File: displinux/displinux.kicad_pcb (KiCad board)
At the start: 2 copper layers, 145 parts, among them J1 USB4105-GF-A, J10 Conn_01x03, J2 USB4105-GF-A, J3 AudioJack4, J4 Conn_02x10_Counter_Clockwise, J5 HR911105A, J6 Conn_01x24_MountingPin, J7 Conn_01x06, J8 Conn_01x40_MountingPin, J9 Conn_01x02_Pin, U1 DP83848C, U2 SY8089AAAC, U3 F133, U4 SY8089AAAC, U5 XC6206P_2_8_MR, U6 XC6206P_1_2_MR, U7 SY7201ABC, U8 W25N01KV, X1 ASE-50MHz, Y1 24M, Y2 Crystal

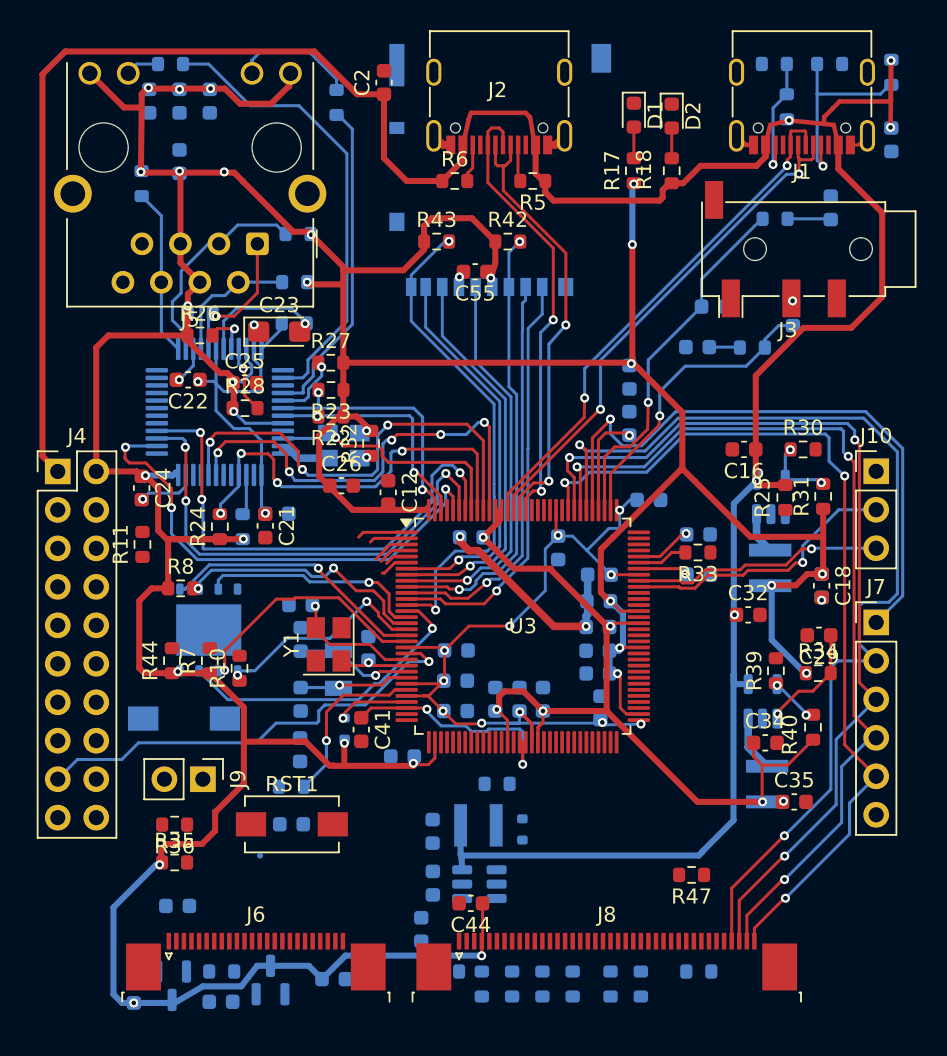
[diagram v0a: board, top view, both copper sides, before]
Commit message: tracing finished Need to check
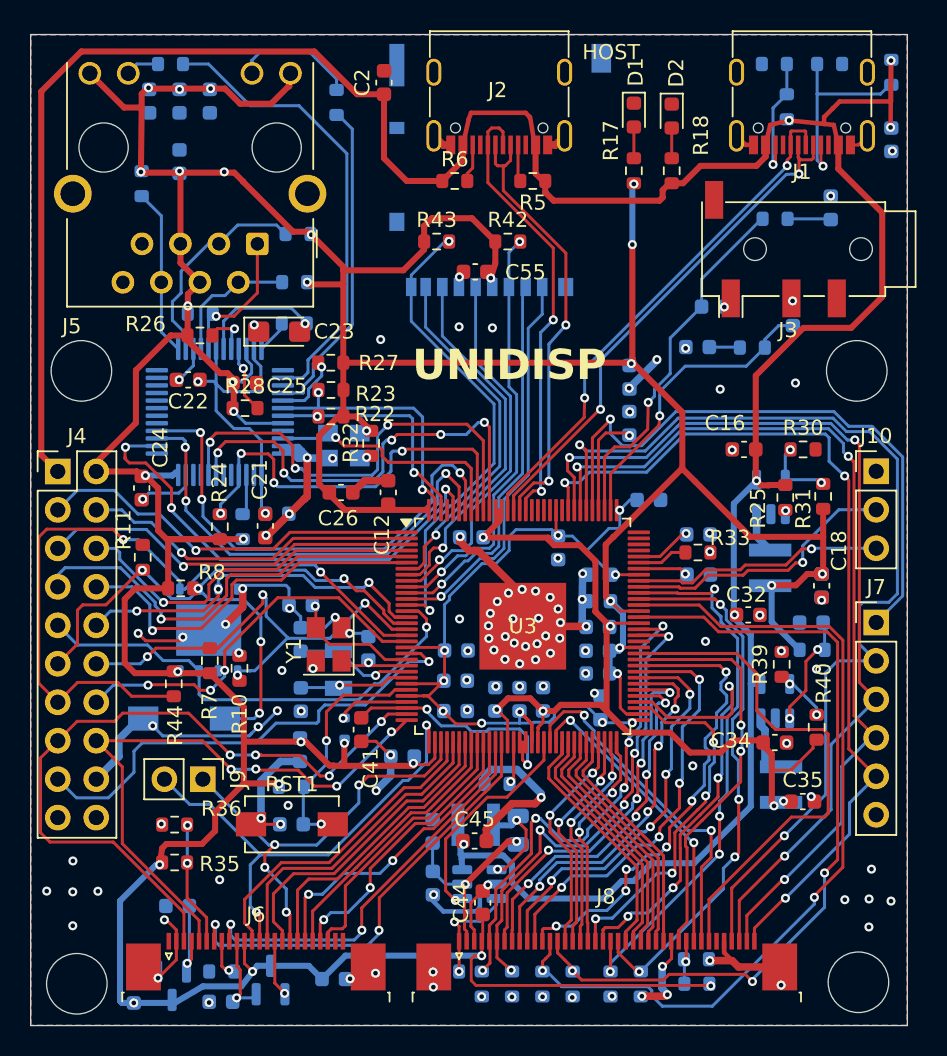
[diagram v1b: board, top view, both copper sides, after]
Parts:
- added ?: , , F.Cu at (246.2, 89.9)
- C29, R34, R47: moved to B.Cu
- C45: moved to F.Cu
- D5: footprint Diode_SMD:D_SOD-523 -> Diode_SMD:D_0805_2012Metric
- moved R47 7.20 mm to (257.7, 113.5)
- moved C45 6.83 mm to (243.0, 104.1), turned to 0 degrees
- moved R34 1.59 mm to (265.3, 91.5)
- moved R44 1.53 mm to (223.1, 93.7), turned to -90 degrees
- moved C29 0.98 mm to (265.2, 89.7)
- moved L2 0.92 mm to (263.2, 100.4)
- moved R11 0.85 mm to (221.1, 85.3)
- moved U4 0.84 mm to (262.8, 94.9)
- moved R48 0.82 mm to (257.6, 111.9)
- moved C44 0.79 mm to (243.5, 108.2), turned to 90 degrees
- moved C34 0.64 mm to (262.8, 97.6)
- moved R39 0.57 mm to (263.3, 92.4)
- moved C35 0.57 mm to (264.7, 101.5)
- moved C26 0.45 mm to (234.2, 81.1)
- moved D5 0.28 mm to (245.9, 103.4)
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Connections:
- J2 pad A1: GND -> (no net)
- J2 pad A12: GND -> (no net)
- J2 pad B1: GND -> (no net)
- J2 pad B12: GND -> (no net)
- U8 pad 9: (no net) -> GND
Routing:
- net GND: track 37.6 -> 143.0 mm, vias 7 -> 120
- net /LCD0-D8: track 0.00 -> 56.8 mm, vias 0 -> 2
- net /LCD0-D9: track 0.00 -> 53.8 mm, vias 0 -> 3
- net /TWI2-SDA: track 0.00 -> 48.3 mm, vias 0 -> 4
- net /TWI2-SCK: track 0.00 -> 39.9 mm, vias 0 -> 4
- net /LCD0-D0: track 0.00 -> 37.2 mm, vias 0 -> 4
- net /LCD0-D1: track 0.00 -> 36.5 mm, vias 0 -> 4
- net /LCD0-DE: track 0.00 -> 34.4 mm
- net /LCD0-D16: track 0.00 -> 34.0 mm, vias 0 -> 5
- net /LCD0-D17: track 0.00 -> 33.0 mm, vias 0 -> 5
- net /NCSI0-MCLK: track 0.00 -> 32.1 mm, vias 0 -> 2
- net /LCD0-D23: track 0.00 -> 32.1 mm, vias 0 -> 6
- net /SPI0_CS0: track 17.7 -> 49.1 mm, vias 1 -> 2
- net /LCD0-D15: track 0.00 -> 30.4 mm, vias 0 -> 4
- net /NCSI0-VSYNC: track 0.00 -> 29.7 mm, vias 0 -> 2
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- added copper zone on B.Cu, net GND
- added copper zone on F.Cu, net GND
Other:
- board outline added: 57.9 x 65.4 mm
- board text added: "+3.3"
- board text added: "+5"
- board text added: "3n"
- board text added: "3p"
- board text added: "HOST"
- board text added: "OTG"
- board text added: "Rx"
- board text added: "Tx"
- board text added: "UNIDISP"
- board text added: "clk"
- board text added: "clk0"
- board text added: "cs0"
- board text added: "g10"
- board text added: "g11"
- board text added: "g6"
- board text added: "g7"
- board text added: "g8"
- board text added: "g9"
- board text added: "gnd"
- board text added: "hold"
- board text added: "iso"
- board text added: "osi"
- board text added: "sck"
- board text added: "sda"
- board text added: "wp"
